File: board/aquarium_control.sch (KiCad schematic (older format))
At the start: 9 parts, among them J1 Barrel_Jack, U1 AP1507

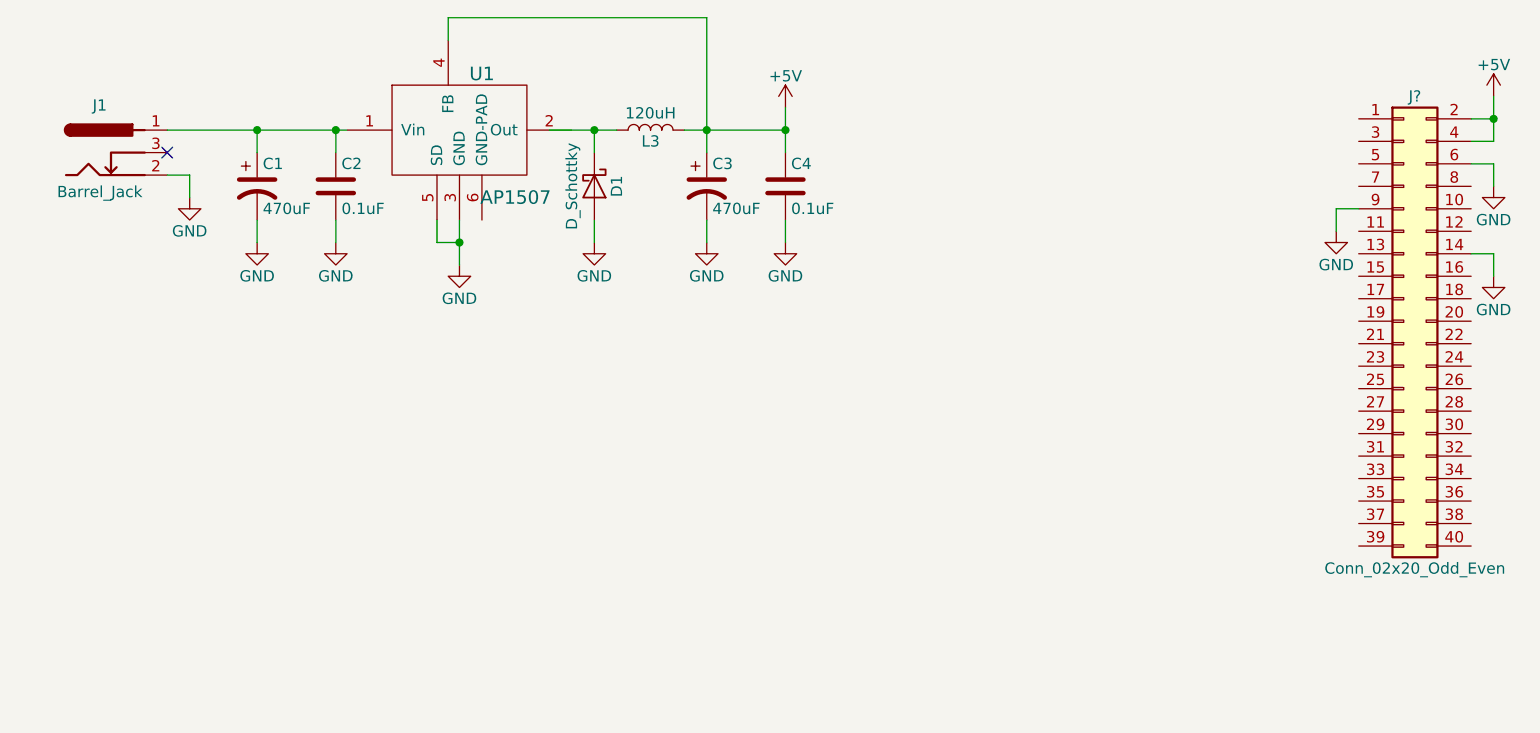
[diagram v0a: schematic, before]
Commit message: Finished power supply design (hopefully)
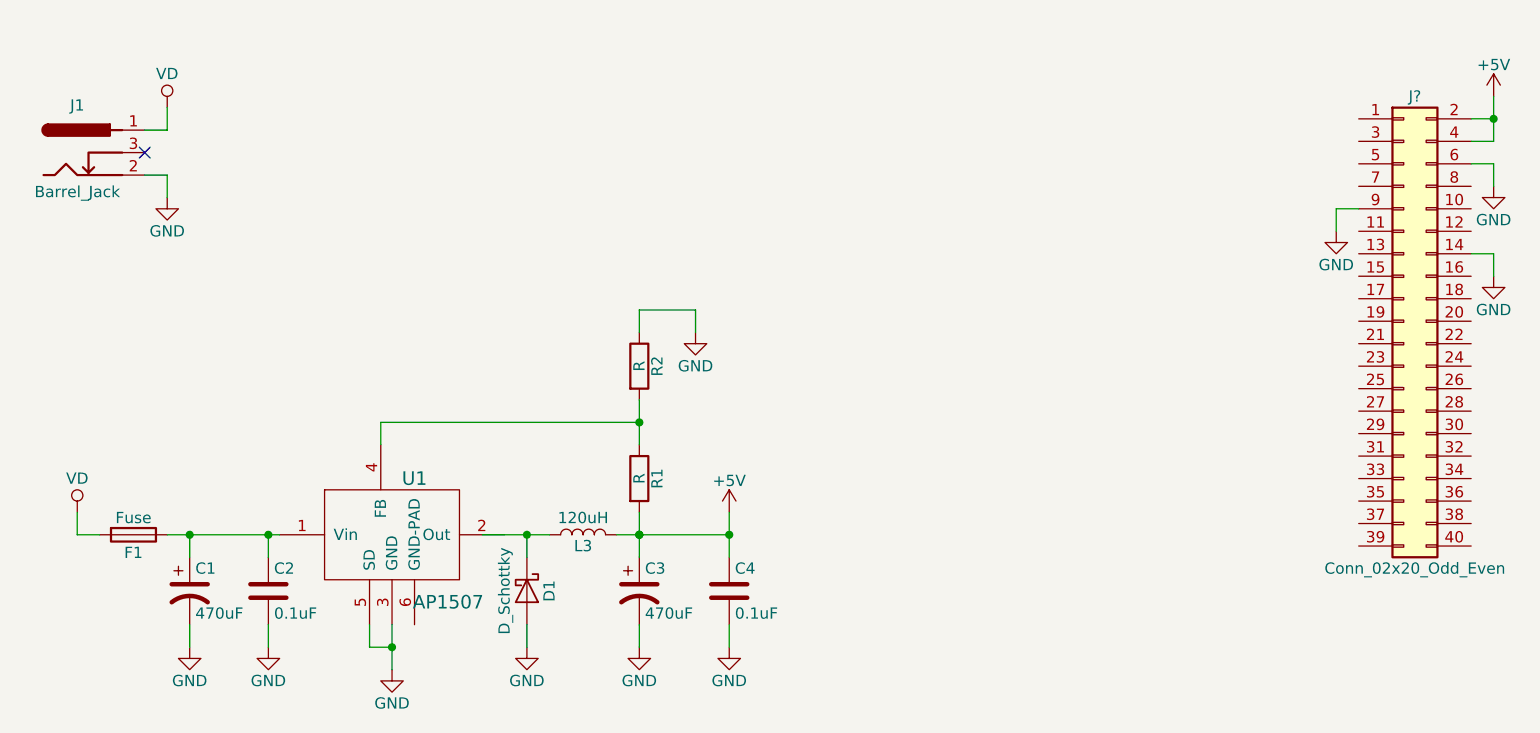
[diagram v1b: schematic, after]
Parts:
- added F1: Fuse, symbol Fuse
- added R1, R2: R, symbol R
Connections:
- net +5V: now also R1.2; no longer U1.4 (FB)
- net GND: now also R2.1
- net at C1.1, C2.1, U1.1 (Vin): now also F1.1; no longer J1.1
- new net: R1.1, R2.2, U1.4 (FB)
- new net VD: F1.2, J1.1
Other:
- moved on the sheet: C1, C2, C3, C4, D1, J1, L3, U1
